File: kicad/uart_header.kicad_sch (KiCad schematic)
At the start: 3 parts, among them J4 Conn_01x07

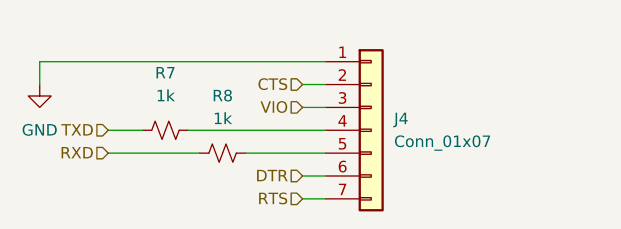
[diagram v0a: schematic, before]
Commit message: blenders
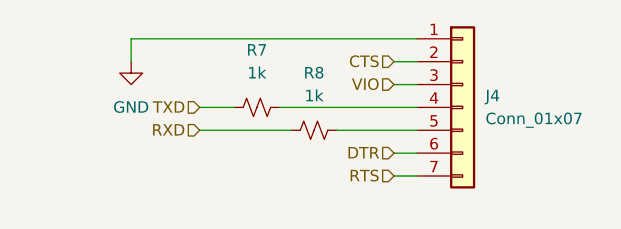
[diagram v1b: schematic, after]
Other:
- moved on the sheet: J4, R7, R8
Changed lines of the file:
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@@
 	(wire
 		(pts
-			(xy 44.45 27.94) (xy 46.99 27.94)
-		)
-		(stroke
-			(width 0)
-			(type default)
-		)
-	)
-	(wire
-		(pts
-			(xy 22.86 33.02) (xy 26.67 33.02)
-		)
-		(stroke
-			(width 0)
-			(type default)
-		)
-	)
-	(wire
-		(pts
-			(xy 44.45 40.64) (xy 46.99 40.64)
-		)
-		(stroke
-			(width 0)
-			(type default)
-		)
-	)
-	(wire
-		(pts
-			(xy 44.45 38.1) (xy 46.99 38.1)
-		)
-		(stroke
-			(width 0)
-			(type default)
-		)
-	)
-	(wire
-		(pts
-			(xy 31.75 33.02) (xy 46.99 33.02)
-		)
-		(stroke
-			(width 0)
-			(type default)
-		)
-	)
-	(wire
-		(pts
-			(xy 22.86 35.56) (xy 33.02 35.56)
-		)
-		(stroke
-			(width 0)
-			(type default)
-		)
-	)
-	(wire
-		(pts
-			(xy 15.24 25.4) (xy 46.99 25.4)
-		)
-		(stroke
-			(width 0)
-			(type default)
-		)
-	)
-	(wire
-		(pts
-			(xy 44.45 30.48) (xy 46.99 30.48)
-		)
-		(stroke
-			(width 0)
-			(type default)
-		)
-	)
-	(wire
-		(pts
-			(xy 15.24 25.4) (xy 15.24 27.94)
-		)
-		(stroke
-			(width 0)
-			(type default)
-		)
-	)
-	(wire
-		(pts
-			(xy 38.1 35.56) (xy 46.99 35.56)
+			(xy 54.61 25.4) (xy 57.15 25.4)
+		)
+		(stroke
+			(width 0)
+			(type default)
+		)
+	)
+	(wire
+		(pts
+			(xy 33.02 30.48) (xy 36.83 30.48)
+		)
+		(stroke
+			(width 0)
+			(type default)
+		)
+	)
+	(wire
+		(pts
+			(xy 54.61 38.1) (xy 57.15 38.1)
+		)
+		(stroke
+			(width 0)
+			(type default)
+		)
+	)
+	(wire
+		(pts
+			(xy 54.61 35.56) (xy 57.15 35.56)
+		)
+		(stroke
+			(width 0)
+			(type default)
+		)
+	)
+	(wire
+		(pts
+			(xy 41.91 30.48) (xy 57.15 30.48)
+		)
+		(stroke
+			(width 0)
+			(type default)
+		)
+	)
+	(wire
+		(pts
+			(xy 33.02 33.02) (xy 43.18 33.02)
+		)
+		(stroke
+			(width 0)
+			(type default)
+		)
+	)
+	(wire
+		(pts
+			(xy 25.4 22.86) (xy 57.15 22.86)
+		)
+		(stroke
+			(width 0)
+			(type default)
+		)
+	)
+	(wire
+		(pts
+			(xy 54.61 27.94) (xy 57.15 27.94)
+		)
+		(stroke
+			(width 0)
+			(type default)
+		)
+	)
+	(wire
+		(pts
+			(xy 25.4 22.86) (xy 25.4 25.4)
+		)
+		(stroke
+			(width 0)
+			(type default)
+		)
+	)
+	(wire
+		(pts
+			(xy 48.26 33.02) (xy 57.15 33.02)
 		)
 		(stroke
@@
 	(hierarchical_label "DTR"
 		(shape input)
-		(at 44.45 38.1 180)
+		(at 54.61 35.56 180)
 		(effects
 			(font
@@
 	(hierarchical_label "RTS"
 		(shape input)
-		(at 44.45 40.64 180)
+		(at 54.61 38.1 180)
 		(effects
 			(font
@@
 	(hierarchical_label "TXD"
 		(shape input)
-		(at 22.86 33.02 180)
+		(at 33.02 30.48 180)
 		(effects
 			(font
@@
 	(hierarchical_label "CTS"
 		(shape input)
-		(at 44.45 27.94 180)
+		(at 54.61 25.4 180)
 		(effects
 			(font
@@
 	(hierarchical_label "RXD"
 		(shape input)
-		(at 22.86 35.56 180)
+		(at 33.02 33.02 180)
 		(effects
 			(font
@@
 	(hierarchical_label "VIO"
 		(shape input)
-		(at 44.45 30.48 180)
+		(at 54.61 27.94 180)
 		(effects
 			(font
@@
 	(symbol
 		(lib_id "power:GND")
-		(at 15.24 27.94 0)
+		(at 25.4 25.4 0)
 		(unit 1)
 		(body_style 1)
@@
 		(fields_autoplaced yes)
 		(property "Reference" "#PWR013"
-			(at 15.24 34.29 0)
+			(at 25.4 31.75 0)
 			(hide yes)
 			(show_name no)
@@
 		)
 		(property "Value" "GND"
-			(at 15.24 33.02 0)
+			(at 25.4 30.48 0)
 			(show_name no)
 			(do_not_autoplace no)
@@
 		)
 		(property "Footprint" ""
-			(at 15.24 27.94 0)
+			(at 25.4 25.4 0)
 			(hide yes)
 			(show_name no)
@@
 		)
 		(property "Datasheet" ""
-			(at 15.24 27.94 0)
+			(at 25.4 25.4 0)
 			(hide yes)
 			(show_name no)
@@
 		)
 		(property "Description" "Power symbol creates a global label with name \"GND\" , ground"
-			(at 15.24 27.94 0)
+			(at 25.4 25.4 0)
 			(hide yes)
 			(show_name no)
@@
 	(symbol
 		(lib_id "Device:R_Small_US")
-		(at 35.56 35.56 90)
+		(at 45.72 33.02 90)
 		(unit 1)
 		(body_style 1)
@@
 		(fields_autoplaced yes)
 		(property "Reference" "R8"
-			(at 35.56 29.21 90)
+			(at 45.72 26.67 90)
 			(show_name no)
 			(do_not_autoplace no)
@@
 		)
 		(property "Value" "1k"
-			(at 35.56 31.75 90)
+			(at 45.72 29.21 90)
 			(show_name no)
 			(do_not_autoplace no)
@@
 		)
 		(property "Footprint" "Resistor_SMD:R_0805_2012Metric_Pad1.20x1.40mm_HandSolder"
-			(at 35.56 35.56 0)
+			(at 45.72 33.02 0)
 			(hide yes)
 			(show_name no)
@@
 		)
 		(property "Datasheet" ""
-			(at 35.56 35.56 0)
+			(at 45.72 33.02 0)
 			(hide yes)
 			(show_name no)
@@
 		)
 		(property "Description" "Resistor, small US symbol"
-			(at 35.56 35.56 0)
+			(at 45.72 33.02 0)
 			(hide yes)
 			(show_name no)
@@
 	(symbol
 		(lib_id "Connector_Generic:Conn_01x07")
-		(at 52.07 33.02 0)
+		(at 62.23 30.48 0)
 		(unit 1)
 		(body_style 1)
@@
 		(fields_autoplaced yes)
 		(property "Reference" "J4"
-			(at 54.61 31.7499 0)
+			(at 64.77 29.2099 0)
 			(show_name no)
 			(do_not_autoplace no)
@@
 		)
 		(property "Value" "Conn_01x07"
-			(at 54.61 34.2899 0)
+			(at 64.77 31.7499 0)
 			(show_name no)
 			(do_not_autoplace no)
@@
 		)
 		(property "Footprint" "Connector_PinHeader_2.54mm:PinHeader_1x07_P2.54mm_Vertical"
-			(at 52.07 33.02 0)
+			(at 62.23 30.48 0)
 			(hide yes)
 			(show_name no)
@@
 		)
 		(property "Datasheet" ""
-			(at 52.07 33.02 0)
+			(at 62.23 30.48 0)
 			(hide yes)
 			(show_name no)
@@
 		)
 		(property "Description" "Generic connector, single row, 01x07, script generated (kicad-library-utils/schlib/autogen/connector/)"
-			(at 52.07 33.02 0)
+			(at 62.23 30.48 0)
 			(hide yes)
 			(show_name no)
@@
 	(symbol
 		(lib_id "Device:R_Small_US")
-		(at 29.21 33.02 90)
+		(at 39.37 30.48 90)
 		(unit 1)
 		(body_style 1)
@@
 		(fields_autoplaced yes)
 		(property "Reference" "R7"
-			(at 29.21 26.67 90)
+			(at 39.37 24.13 90)
 			(show_name no)
 			(do_not_autoplace no)
@@
 		)
 		(property "Value" "1k"
-			(at 29.21 29.21 90)
+			(at 39.37 26.67 90)
 			(show_name no)
 			(do_not_autoplace no)
@@
 		)
 		(property "Footprint" "Resistor_SMD:R_0805_2012Metric_Pad1.20x1.40mm_HandSolder"
-			(at 29.21 33.02 0)
+			(at 39.37 30.48 0)
 			(hide yes)
 			(show_name no)
@@
 		)
 		(property "Datasheet" ""
-			(at 29.21 33.02 0)
+			(at 39.37 30.48 0)
 			(hide yes)
 			(show_name no)
@@
 		)
 		(property "Description" "Resistor, small US symbol"
-			(at 29.21 33.02 0)
-			(hide yes)
-			(show_name no)
+			(at 39.37 30.48 0)
+			(hide yes)
+			(show_name no)
